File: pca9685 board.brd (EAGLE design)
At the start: 27.3 x 38.7 mm, 4 parts

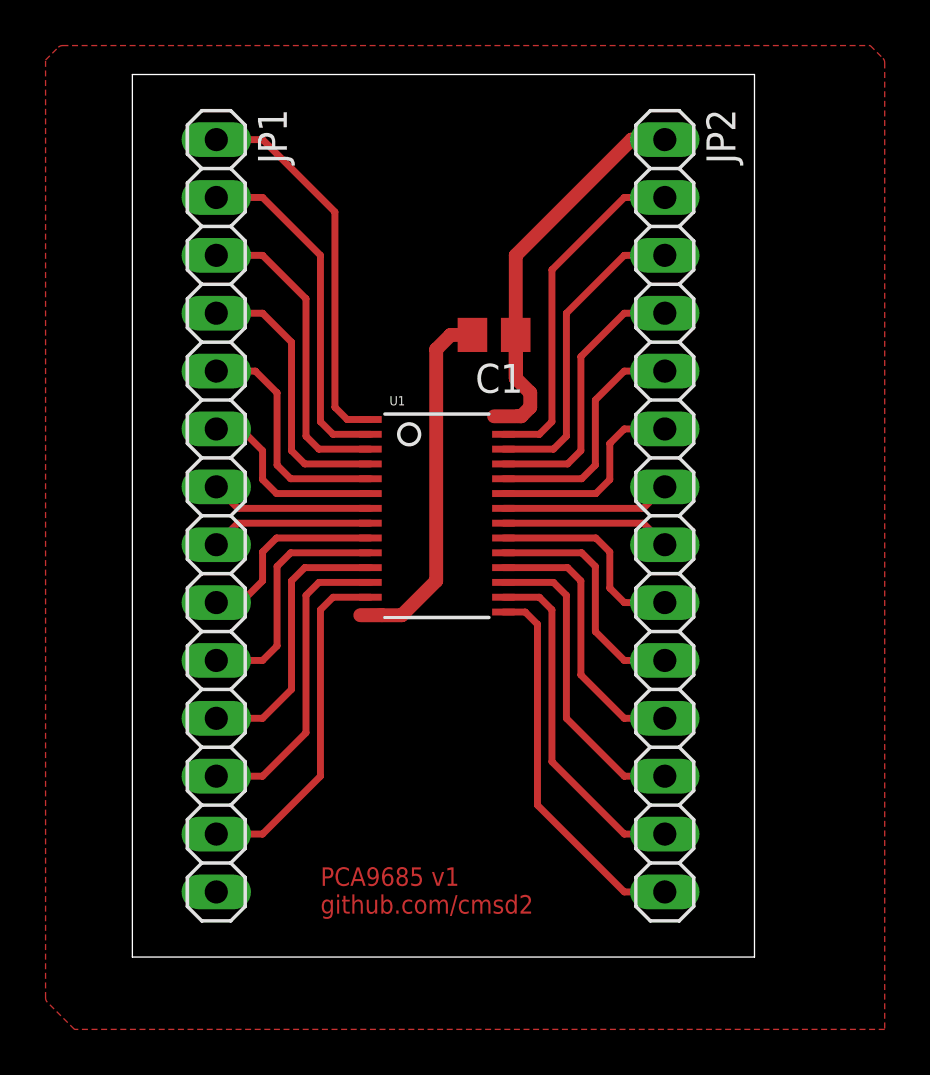
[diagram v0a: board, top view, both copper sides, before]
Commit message: don't really need such fat power lines
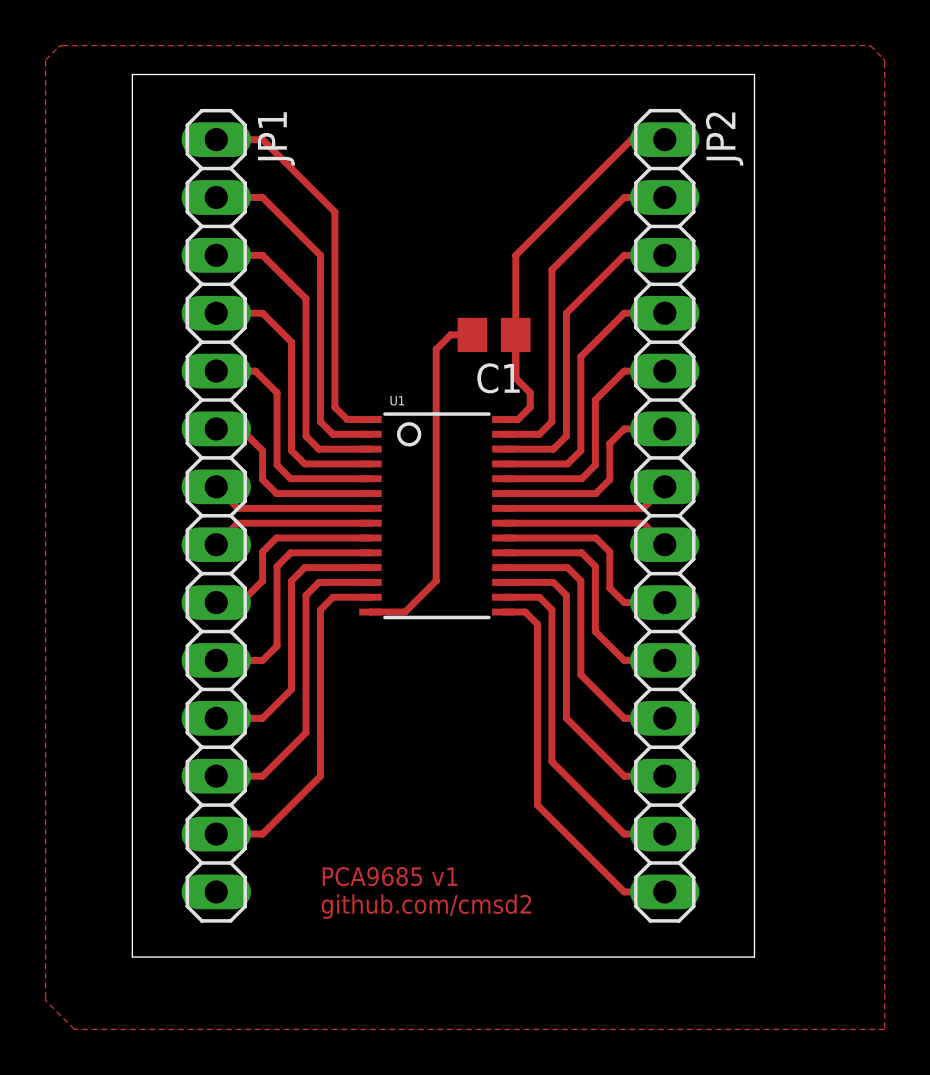
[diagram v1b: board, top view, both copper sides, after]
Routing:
- net GND: track 16.5 -> 15.5 mm
- net N$2: track 0.95 -> 0.00 mm
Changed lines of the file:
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@@
 <setting verticaltext="up"/>
 </settings>
-<grid distance="0.025" unitdist="inch" unit="inch" style="lines" multiple="1" display="yes" altdistance="0.00625" altunitdist="inch" altunit="inch"/>
+<grid distance="0.0125" unitdist="inch" unit="inch" style="lines" multiple="1" display="yes" altdistance="0.003125" altunitdist="inch" altunit="inch"/>
 <layers>
 <layer number="1" name="Top" color="4" fill="1" visible="yes" active="yes"/>
@@
 <layer number="39" name="tKeepout" color="4" fill="11" visible="no" active="yes"/>
 <layer number="40" name="bKeepout" color="1" fill="11" visible="no" active="yes"/>
-<layer number="41" name="tRestrict" color="4" fill="10" visible="no" active="yes"/>
+<layer number="41" name="tRestrict" color="4" fill="10" visible="yes" active="yes"/>
 <layer number="42" name="bRestrict" color="1" fill="10" visible="no" active="yes"/>
 <layer number="43" name="vRestrict" color="2" fill="10" visible="no" active="yes"/>
@@
 <wire x1="-0.635" y1="38.1" x2="-0.635" y2="-0.635" width="0" layer="20"/>
 <polygon width="0.0254" layer="41" pour="hatch">
-<vertex x="8.73125" y="14.9225"/>
-<vertex x="10.795" y="14.9225"/>
-<vertex x="12.065" y="16.1925"/>
-<vertex x="12.065" y="26.3525"/>
-<vertex x="13.17625" y="27.46375"/>
-<vertex x="13.49375" y="27.46375"/>
-<vertex x="13.49375" y="25.7175"/>
-<vertex x="13.335" y="24.13"/>
-<vertex x="13.335" y="15.5575"/>
-<vertex x="11.509375" y="13.731875"/>
-<vertex x="8.73125" y="13.731875"/>
+<vertex x="9.04875" y="14.9225"/>
+<vertex x="10.9809875" y="14.9225" curve="45"/>
+<vertex x="11.20549375" y="15.01549375"/>
+<vertex x="12.13075625" y="15.94075625" curve="45"/>
+<vertex x="12.22375" y="16.1652625"/>
+<vertex x="12.22375" y="26.0622375" curve="-45"/>
+<vertex x="12.31674375" y="26.28674375"/>
+<vertex x="13.08325625" y="27.05325625" curve="-45"/>
+<vertex x="13.3077625" y="27.14625"/>
+<vertex x="13.49375" y="27.14625"/>
+<vertex x="13.49375" y="26.19375"/>
+<vertex x="13.1699" y="25.87625"/>
+<vertex x="13.17625" y="24.892"/>
+<vertex x="13.17625" y="15.8477625" curve="-45"/>
+<vertex x="13.08325625" y="15.62325625"/>
+<vertex x="11.60236875" y="14.14236875" curve="-45"/>
+<vertex x="11.3778625" y="14.049375"/>
+<vertex x="9.36625" y="14.049375" curve="-90"/>
+<vertex x="9.04875" y="14.366875"/>
 </polygon>
 <text x="7.62" y="1.27" size="0.8128" layer="1" font="vector">PCA9685 v1
@@
 <contactref element="JP2" pad="1"/>
 <contactref element="C1" pad="1"/>
-<wire x1="16.19" y1="26.67" x2="16.1925" y2="24.7675" width="0.6096" layer="1"/>
-<wire x1="16.1925" y1="24.7675" x2="16.1925" y2="30.1625" width="0.6096" layer="1"/>
-<wire x1="16.1925" y1="30.1625" x2="21.2725" y2="35.2425" width="0.6096" layer="1"/>
-<wire x1="21.2725" y1="35.2425" x2="22.733" y2="35.2425" width="0.6096" layer="1"/>
-<wire x1="16.1925" y1="24.7675" x2="16.8275" y2="24.1325" width="0.6096" layer="1"/>
-<wire x1="16.8275" y1="24.1325" x2="16.8275" y2="23.495" width="0.6096" layer="1"/>
-<wire x1="16.8275" y1="23.495" x2="16.430625" y2="23.098125" width="0.6096" layer="1"/>
-<wire x1="16.430625" y1="23.098125" x2="16.271875" y2="23.098125" width="0.6096" layer="1"/>
-<wire x1="16.271875" y1="23.098125" x2="16.13125" y2="22.9575" width="0.3048" layer="1"/>
-<wire x1="16.13125" y1="22.9575" x2="15.64955" y2="22.9575" width="0.3048" layer="1"/>
+<wire x1="16.19" y1="26.67" x2="16.1925" y2="24.7675" width="0.3048" layer="1"/>
+<wire x1="16.1925" y1="24.7675" x2="16.1925" y2="30.1625" width="0.3048" layer="1"/>
+<wire x1="16.1925" y1="30.1625" x2="21.2725" y2="35.2425" width="0.3048" layer="1"/>
+<wire x1="21.2725" y1="35.2425" x2="22.733" y2="35.2425" width="0.3048" layer="1"/>
+<wire x1="16.1925" y1="24.7675" x2="16.8275" y2="24.1325" width="0.3048" layer="1"/>
+<wire x1="16.8275" y1="24.1325" x2="16.8275" y2="23.495" width="0.3048" layer="1"/>
+<wire x1="15.64955" y1="22.9575" x2="16.29" y2="22.9575" width="0.3048" layer="1"/>
+<wire x1="16.29" y1="22.9575" x2="16.8275" y2="23.495" width="0.3048" layer="1"/>
 </signal>
 <signal name="SDA">
@@
 <contactref element="U1" pad="14"/>
 <contactref element="C1" pad="2"/>
-<wire x1="12.7" y1="26.035" x2="12.7" y2="15.875" width="0.6096" layer="1"/>
-<wire x1="12.7" y1="15.875" x2="11.191875" y2="14.366875" width="0.6096" layer="1"/>
+<wire x1="12.7" y1="26.035" x2="12.7" y2="15.875" width="0.3048" layer="1"/>
+<wire x1="12.7" y1="15.875" x2="11.337921875" y2="14.510384375" width="0.3048" layer="1"/>
 <polygon width="0.254" layer="1" rank="2">
 <vertex x="-4.445" y="38.735"/>
@@
 <vertex x="-4.445" y="-2.434790625"/>
 </polygon>
-<wire x1="12.7" y1="26.035" x2="13.335" y2="26.67" width="0.6096" layer="1"/>
-<wire x1="13.335" y1="26.67" x2="14.29" y2="26.67" width="0.6096" layer="1"/>
-<wire x1="11.191875" y1="14.366875" x2="10.31875" y2="14.366875" width="0.6096" layer="1"/>
-<wire x1="10.31875" y1="14.366875" x2="10.178125" y2="14.5075" width="0.3048" layer="1"/>
-<wire x1="10.178125" y1="14.5075" x2="9.81395" y2="14.5075" width="0.3048" layer="1"/>
-<wire x1="10.31875" y1="14.366875" x2="9.36625" y2="14.366875" width="0.6096" layer="1"/>
+<wire x1="12.7" y1="26.035" x2="13.335" y2="26.67" width="0.3048" layer="1"/>
+<wire x1="13.335" y1="26.67" x2="14.29" y2="26.67" width="0.3048" layer="1"/>
+<wire x1="11.337921875" y1="14.510384375" x2="9.81395" y2="14.50784375" width="0.3048" layer="1"/>
+<wire x1="9.81395" y1="14.50784375" x2="9.81395" y2="14.5075" width="0.3048" layer="1"/>
 </signal>
 <signal name="PWM0">
@@
 <signal name="N$1">
 </signal>
-<signal name="N$2">
-<wire x1="16.1925" y1="23.098125" x2="15.24" y2="23.098125" width="0.6096" layer="1"/>
-</signal>
 </signals>
